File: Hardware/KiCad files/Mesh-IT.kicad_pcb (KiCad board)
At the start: 4 copper layers, 150 x 110 mm, 94 parts, among them Q1 SS8050, SW1 SW_Push, SW10 SW_Push, SW11 SW_Push, SW12 SW_Push, SW13 SW_Push, SW14 SW_Push, SW15 SW_Push, SW16 SW_Push, SW17 SW_Push, SW18 SW_Push, SW19 SW_Push, SW2 SW_Push, SW20 SW_Push, SW21 SW_Push, SW22 SW_Push, SW23 SW_Push, SW24 SW_Push, SW25 SW_Push, SW26 SW_Push, SW27 SW_Push, SW28 SW_Push, SW29 SW_Push, SW3 SW_Push, SW30 SW_Push, SW31 SW_Push, SW32 SW_Push, SW33 SW_Push, SW34 SW_Push, SW35 SW_Push, SW4 SW_Push, SW5 SW_Push, SW6 SW_Push, SW7 SW_Push, SW8 SW_Push, SW9 SW_Push, U1 XIAO-ESP32-S3-DIP

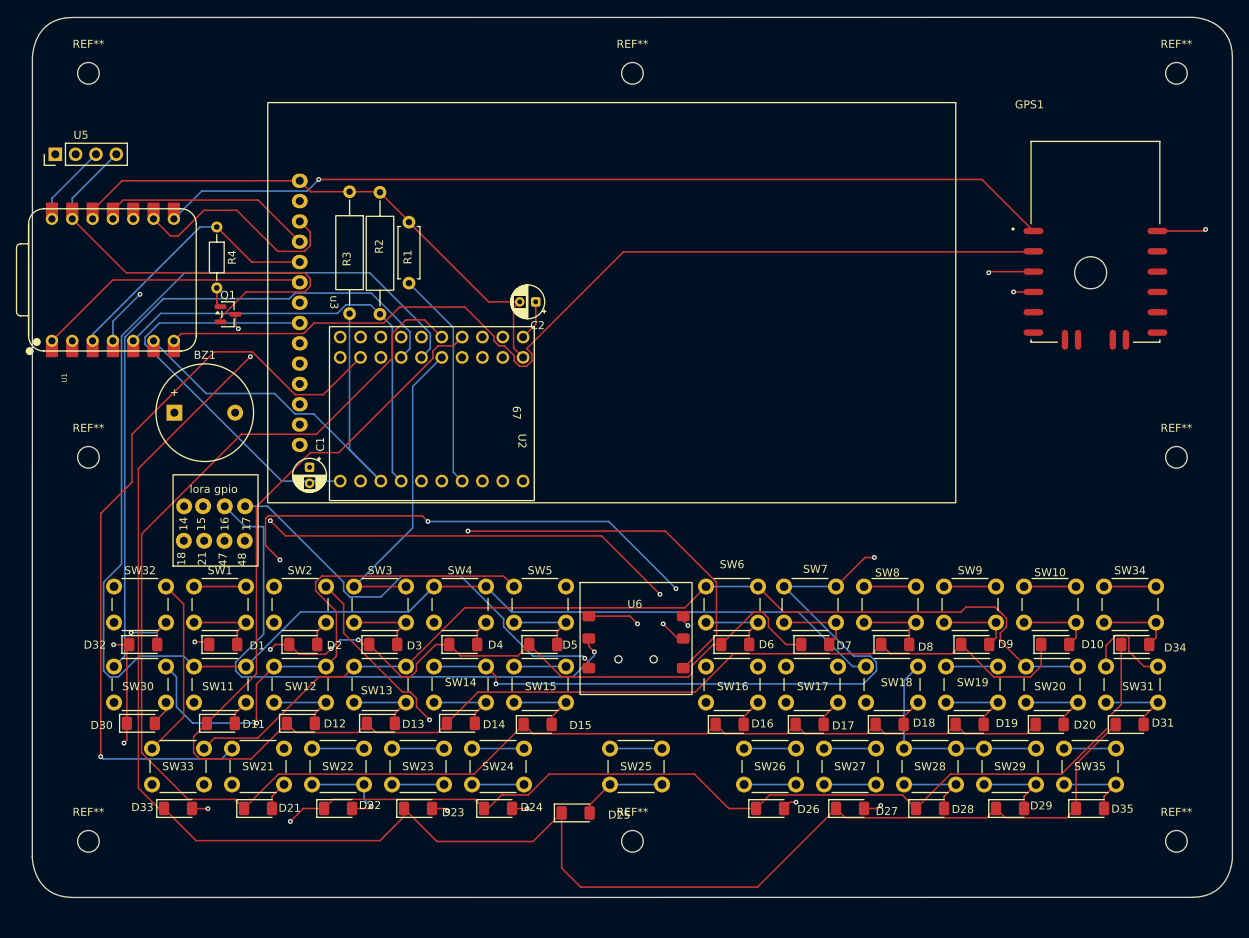
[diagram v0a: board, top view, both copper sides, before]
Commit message: Uploading final files
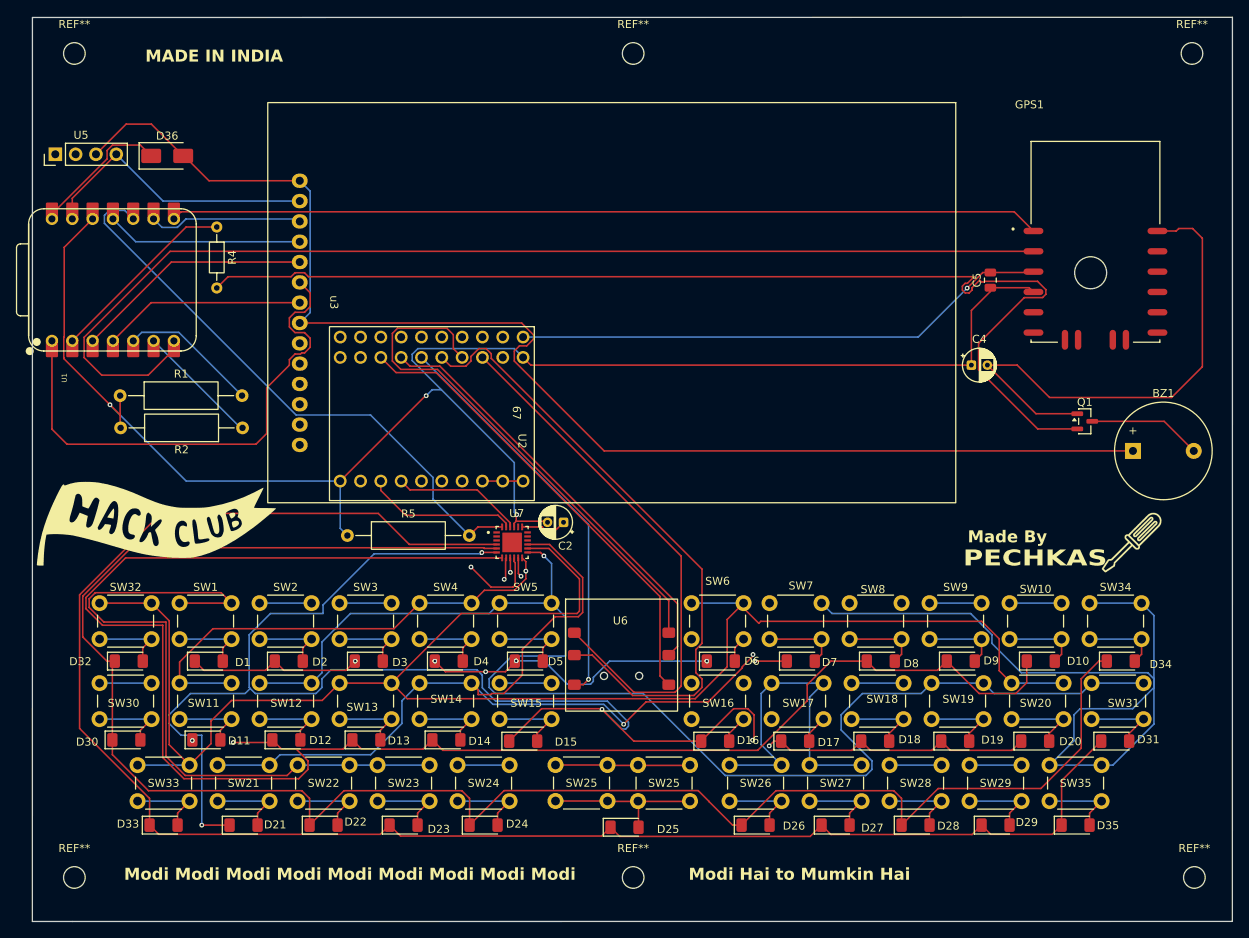
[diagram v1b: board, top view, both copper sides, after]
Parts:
- removed C1: 0.1uf, Capacitor_THT:CP_Radial_D4.0mm_P2.00mm
- removed R3: 4.7K, Resistor_THT:R_Axial_DIN0309_L9.0mm_D3.2mm_P15.24mm_Horizontal
- removed the REF** at (116.8, 210.5)
- removed the REF** at (252.8, 210.5)
- removed the REF** at (184.8, 114.5)
- removed the REF** at (252.8, 114.5)
- removed the REF** at (116.8, 162.5)
- removed the REF** at (184.8, 210.5)
- removed the REF** at (252.8, 162.5)
- removed the REF** at (116.8, 114.5)
- removed U4: ~, XIAO S3:Lora hat gpio pins
- added .: LOGO, LOGO, F.Cu at (247.2, 173.1)
- added .: LOGO, LOGO, B.Cu at (161.1, 131.0)
- added C4: 0.1uf, Capacitor_THT:CP_Radial_D4.0mm_P2.00mm, F.Cu at (227.1, 151.0)
- added C5: 10uf, Capacitor_SMD:C_0805_2012Metric, F.Cu at (229.5, 140.3)
- added D36: SS14, Diode_SMD:D_SMA, F.Cu at (126.6, 124.8)
- added G***: LOGO, LOGO, F.Cu at (125.3, 170.8)
- added R5: 4.7K, Resistor_THT:R_Axial_DIN0309_L9.0mm_D3.2mm_P15.24mm_Horizontal, F.Cu at (149.1, 172.3)
- added REF**: MountingHole_2.7mm_M2.5, MountingHole:MountingHole_2.7mm_M2.5, F.Cu at (115.0, 112.0)
- added REF**: MountingHole_2.7mm_M2.5, MountingHole:MountingHole_2.7mm_M2.5, F.Cu at (115.0, 215.0)
- added REF**: MountingHole_2.7mm_M2.5, MountingHole:MountingHole_2.7mm_M2.5, F.Cu at (184.8, 215.0)
- added REF**: MountingHole_2.7mm_M2.5, MountingHole:MountingHole_2.7mm_M2.5, F.Cu at (255.0, 215.0)
- added REF**: MountingHole_2.7mm_M2.5, MountingHole:MountingHole_2.7mm_M2.5, F.Cu at (254.7, 112.0)
- added REF**: MountingHole_2.7mm_M2.5, MountingHole:MountingHole_2.7mm_M2.5, F.Cu at (184.8, 112.0)
- added SW25: SW_Push, Button_Switch_THT:SW_PUSH_6mm_H8mm, F.Cu at (185.5, 200.9)
- added U7: TCA8418RTWR, XIAO S3:QFN50P400X400X80-25N, F.Cu at (169.7, 173.1)
- R1: value 10K -> 4.7K; footprint Resistor_THT:R_Axial_DIN0207_L6.3mm_D2.5mm_P7.62mm_Horizontal -> Resistor_THT:R_Axial_DIN0309_L9.0mm_D3.2mm_P15.24mm_Horizontal
- R2: value 4.7K -> 4.7k
- moved BZ1 119.9 mm to (247.3, 161.7)
- moved Q1 107.9 mm to (241.3, 158.0)
- moved R1 38.7 mm to (120.7, 154.8), turned to 0 degrees
- moved R2 34.1 mm to (136.0, 158.8), turned to 180 degrees
- moved C2 27.8 mm to (176.1, 170.6)
- moved SW25 7.12 mm to (175.1, 200.9)
- moved D25 6.37 mm to (183.8, 208.7)
- moved D1 2.75 mm to (131.8, 188.0)
- moved D10 2.75 mm to (235.8, 188.0)
- moved D11 2.75 mm to (131.5, 197.8)
- moved D12 2.75 mm to (141.5, 197.8)
- moved D13 2.75 mm to (151.5, 197.8)
- moved D14 2.75 mm to (161.5, 197.8)
- moved D15 2.75 mm to (171.1, 198.0)
- moved D16 2.75 mm to (195.1, 198.0)
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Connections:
- Q1 pad 1: Net-(Q1-B) -> GND
- Q1 pad 2: GND -> Net-(Q1-E)
- R1 pad 1: Net-(U2-RST) -> 3.3V
- R1 pad 2: 3.3V -> I2c_Sda
- R2 pad 1: 3.3V -> SCL_SCK
- R2 pad 2: I2c_Sda -> 3.3V
- R4 pad 1: D2 -> D1
- R4 pad 2: Net-(Q1-B) -> Net-(Q1-E)
- U1 pad 10: unconnected-(U1-GPIO8/D9/A9/MISO-Pad10) -> D9
- U1 pad 14: 5V -> VBUS
- U2 pad 10: Row 3 -> unconnected-(U2-A2-Pad10)
- U2 pad 11: Col 4 -> JOY_RIGHT
- U2 pad 12: Row 4 -> unconnected-(U2-A3-Pad12)
- U2 pad 13: Col 5 -> JOY_PRESS
- U2 pad 14: Row 5 -> unconnected-(U2-A4-Pad14)
- U2 pad 15: Col 6 -> B7
- U2 pad 17: Col 7 -> unconnected-(U2-B6-Pad17)
- U2 pad 19: B7 -> unconnected-(U2-B7-Pad19)
- U2 pad 24: Net-(U2-RST) -> unconnected-(U2-RST-Pad24)
- U2 pad 5: Col 1 -> JOY_UP
- U2 pad 6: Row 1 -> unconnected-(U2-A0-Pad6)
- U2 pad 7: Col 2 -> JOY_DOWN
- U2 pad 8: Row 2 -> unconnected-(U2-A1-Pad8)
- U2 pad 9: Col 3 -> JOY_LEFT
- u3 pad 1: 3.3V -> 5V
- u3 pad 8: 3.3V -> 5V
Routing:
- net Net-(Q1-E): track 0.00 -> 140.3 mm
- net 5V: track 46.7 -> 165.5 mm
- net B7: track 170.5 -> 58.8 mm, vias 1 -> 0
- net GND: track 81.4 -> 190.5 mm, vias 2 -> 1
- net Col 5: track 276.8 -> 193.3 mm
- net JOY_DOWN: track 139.5 -> 65.9 mm, vias 1 -> 0
- net D9: track 0.00 -> 73.2 mm
- net Col 4: track 230.7 -> 164.4 mm, vias 0 -> 1
- net Row 1: track 152.0 -> 95.3 mm, vias 4 -> 7
- net Col 7: track 279.5 -> 230.1 mm, vias 3 -> 2
- net 3.3V: track 248.0 -> 208.8 mm, vias 1 -> 3
- net Col 3: track 190.5 -> 153.2 mm, vias 0 -> 1
- net Row 2: track 189.0 -> 223.9 mm, vias 0 -> 2
- net D0: track 34.3 -> 65.1 mm
- net JOY_PRESS: track 82.4 -> 54.2 mm, vias 4 -> 0
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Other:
- board size 150 x 110 mm -> 150 x 113 mm
- board text added: "MADE IN INDIA"
- board text added: "Made By"
- board text added: "Modi Hai to Mumkin Hai"
- board text added: "Modi Modi Modi Modi Modi Modi Modi Modi Modi"
- board text added: "PECHKAS"
